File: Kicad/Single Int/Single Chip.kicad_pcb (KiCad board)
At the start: 2 copper layers, 51.3 x 38.1 mm, 3 parts, among them J1 Raspberry_Pi_2_3, J2 Conn_01x02, U1 8088_Min_Mode

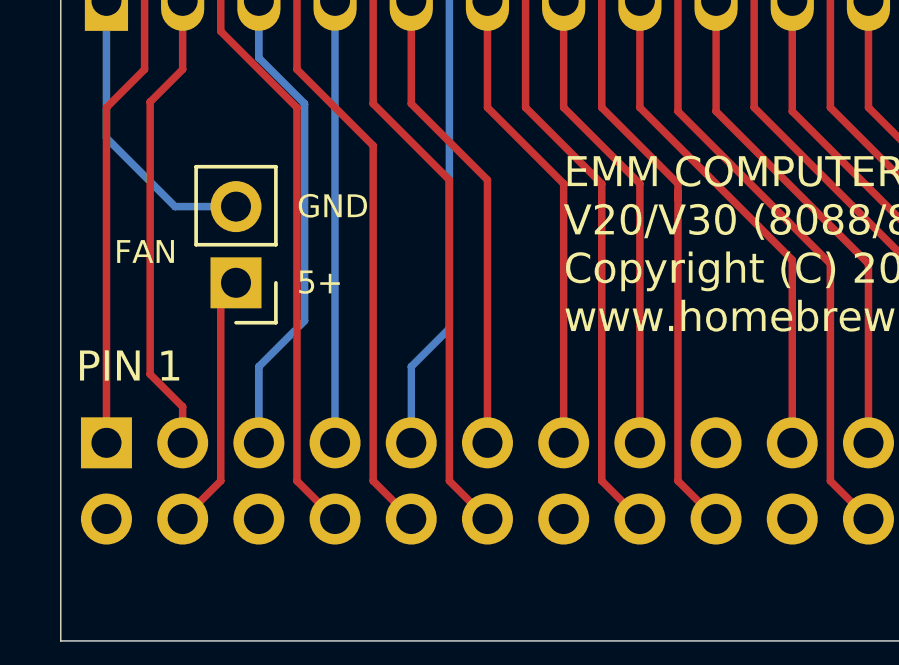
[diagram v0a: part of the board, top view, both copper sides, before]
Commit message: UPDATE
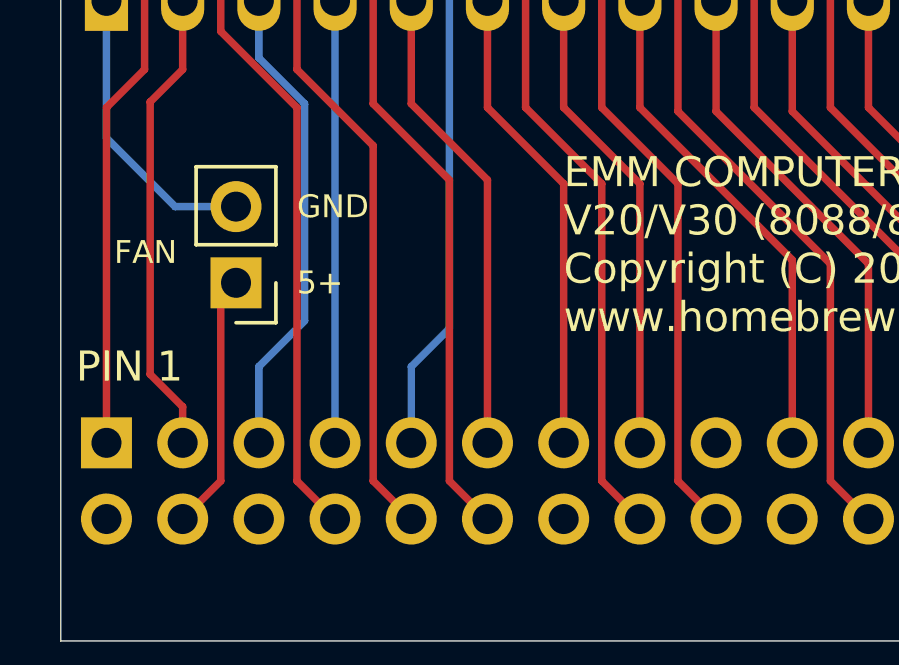
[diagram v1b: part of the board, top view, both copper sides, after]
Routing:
- net /5+: track 8.61 -> 7.89 mm
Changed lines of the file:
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@@
   (segment (start 128.27 96.266) (end 127 97.536) (width 0.25) (layer "F.Cu") (net 1))
   (segment (start 128.27 90.17) (end 128.27 96.266) (width 0.25) (layer "F.Cu") (net 1))
-  (segment (start 128.778 89.662) (end 128.27 90.17) (width 0.25) (layer "F.Cu") (net 1))
   (segment (start 147.32 76.073) (end 147.32 65.024) (width 0.25) (layer "F.Cu") (net 2))
   (segment (start 172.72 80.264) (end 172.72 94.996) (width 0.25) (layer "F.Cu") (net 2))
@@
   (segment (start 140.97 86.36) (end 140.97 96.266) (width 0.25) (layer "F.Cu") (net 5))
   (segment (start 140.97 73.533) (end 137.16 69.723) (width 0.25) (layer "F.Cu") (net 6))
-  (segment (start 143.51 86.868) (end 143.51 86.36) (width 0.25) (layer "F.Cu") (net 6))
-  (segment (start 143.51 96.266) (end 143.51 86.614) (width 0.25) (layer "F.Cu") (net 6))
+  (segment (start 143.51 96.266) (end 143.51 86.36) (width 0.25) (layer "F.Cu") (net 6))
   (segment (start 144.78 97.536) (end 143.51 96.266) (width 0.25) (layer "F.Cu") (net 6))
   (segment (start 143.51 86.36) (end 140.97 83.82) (width 0.25) (layer "F.Cu") (net 6))
